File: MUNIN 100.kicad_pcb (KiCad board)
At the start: 2 copper layers, 100 x 75 mm, 78 parts, among them IC1 ACHS-7123, J1 TX_IN, J2 Conn_Coaxial, J3 Conn_01x03_Male, J4 3-647630-4, Q1 ISS55EP06LMXTSA1, Q2 MRF101AN, Q3 MRF101BN, U1 TL783CKTT, U2 LM358

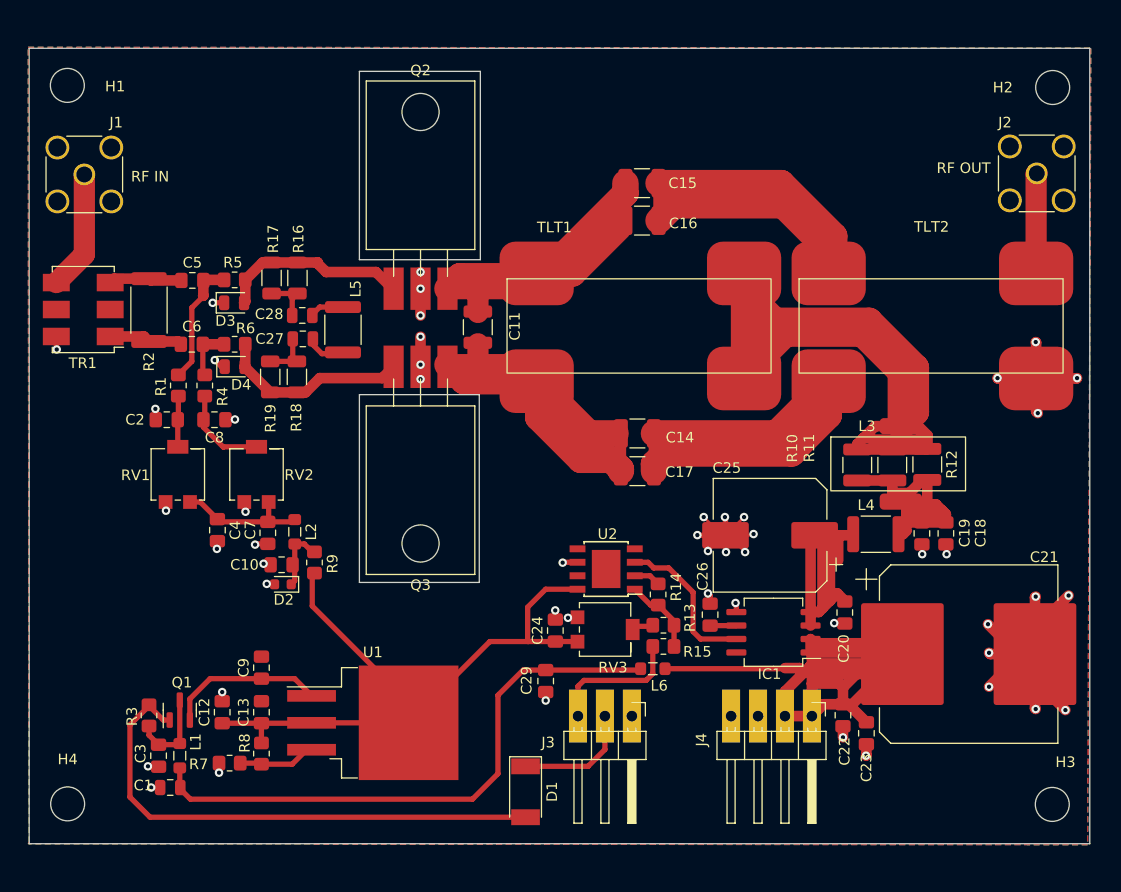
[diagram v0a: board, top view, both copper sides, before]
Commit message: first pcb release
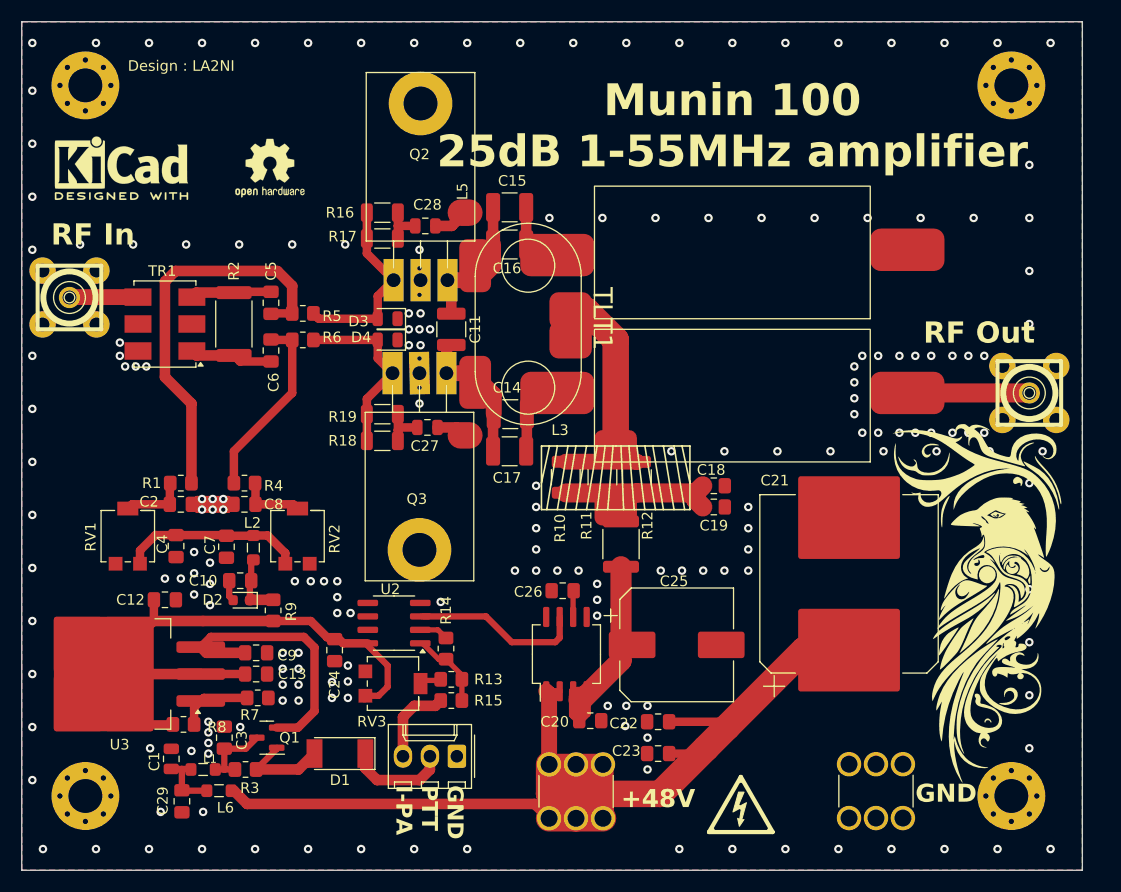
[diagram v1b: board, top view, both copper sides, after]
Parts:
- removed U1: TL783CKTT, Package_TO_SOT_SMD:TO-263-3_TabPin2
- added G***: LOGO, Munin_logo:Munin, F.Cu at (135.0, 130.0)
- added J5: Conn_01x01_Pin, 7461057:7461057, F.Cu at (123.0, 150.1)
- added REF**: OSHW-Logo2_7.3x6mm_SilkScreen, Symbol:OSHW-Logo2_7.3x6mm_SilkScreen, F.Cu at (68.4, 88.8)
- added REF**: Symbol_HighVoltage_Triangle_6x6mm_Copper, logo:Symbol_HighVoltage_Triangle_6x6mm_Copper, F.Cu at (112.8, 148.8)
- added REF**: KiCad-Logo2_5mm_SilkScreen, Symbol:KiCad-Logo2_5mm_SilkScreen, F.Cu at (54.4, 88.8)
- added U3: TL783, Package_TO_SOT_SMD:TO-263-3_TabPin2, F.Cu at (54.2, 136.5)
- H1, H2, H3, H4: value MH -> MountingHole_Pad; footprint MountingHole:MountingHole_3.2mm_M3 -> MountingHole:MountingHole_3.2mm_M3_Pad_Via
- J1, J2: footprint Connector_Coaxial:SMA_Amphenol_132291_Vertical -> SMA_PINS:SMA_PINS
- J3: footprint Connector_PinHeader_2.54mm:PinHeader_1x03_P2.54mm_Horizontal -> Connector_Molex:Molex_KK-254_AE-6410-03A_1x03_P2.54mm_Vertical
- J4: value 3-647630-4 -> Conn_01x01_Pin; footprint Connector_PinHeader_2.54mm:PinHeader_1x04_P2.54mm_Horizontal -> 7461057:7461057
- L1: value L_Core_Ferrite_Small -> 742792096
- L2: value FB -> Wurth: 742792096
- L3: value L_Core_Iron -> FT-50-43; footprint LA2NI:FT_50_1 -> T50:T50_V_smd
- L4: value Ferrite Bead 742792514 -> HI1806T600R-10
- L5: footprint Inductor_SMD:L_1812_4532Metric -> Resistor_THT:R_Axial_DIN0918_L18.0mm_D9.0mm_P30.48mm_Horizontal
- TLT1: value TLT -> FT94-61; footprint LA2NI:TLT_94_3 -> TLT:TLT
- TLT2: value TLT -> FT94-61; footprint LA2NI:TLT_94_3 -> Amidon_Binocular:Dual_FB-61-4852
- U2: footprint Package_SO:Diodes_PSOP-8 -> Package_SO:SOIC-8_3.9x4.9mm_P1.27mm
- moved L6 42.5 mm to (63.6, 147.5)
- moved C29 36.1 mm to (60.1, 148.5)
- moved R10 27.5 mm to (96.3, 117.9)
- moved R12 27.4 mm to (103.0, 118.0)
- moved R11 27.4 mm to (99.8, 117.9)
- moved L3 27.3 mm to (101.0, 118.0)
- moved C20 26.1 mm to (98.6, 140.9), turned to 180 degrees
- moved L4 24.0 mm to (101.5, 124.2), turned to -90 degrees
- moved C18 22.3 mm to (110.2, 118.8), turned to 180 degrees
- moved C24 20.9 mm to (74.5, 134.2), turned to -90 degrees
- moved J2 20.7 mm to (140.0, 110.0), turned to 180 degrees
- moved R13 20.6 mm to (85.5, 137.0)
- moved R14 20.6 mm to (85.0, 134.1)
- moved R15 20.6 mm to (85.5, 139.0)
- moved RV3 20.6 mm to (80.0, 137.4)
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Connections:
- C21 pad 1: Net-(C21-Pad1) -> Net-(J4-Pin_1)
- C22 pad 1: Net-(C21-Pad1) -> Net-(J4-Pin_1)
- C23 pad 1: Net-(C21-Pad1) -> Net-(J4-Pin_1)
- IC1 pad 1: Net-(C21-Pad1) -> Net-(J4-Pin_1)
- IC1 pad 2: Net-(C21-Pad1) -> Net-(J4-Pin_1)
- J4 pad 1: Net-(C21-Pad1) -> Net-(J4-Pin_1)
- L6 pad 2: Net-(C21-Pad1) -> Net-(J4-Pin_1)
- Q2 pad : (no net) -> GND
- Q3 pad : (no net) -> GND
- RV2 pad 1: Net-(C4-Pad1) -> GND
- RV2 pad 3: GND -> Net-(C4-Pad1)
- TLT2 pad 1: Net-(C15-Pad2) -> Net-(C14-Pad2)
- TLT2 pad 4: Net-(C14-Pad2) -> Net-(C15-Pad2)
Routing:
- net Net-(J4-Pin_1): track 0.00 -> 120.6 mm
- net Net-(C21-Pad1): track 87.1 -> 0.00 mm
- net GND: track 106.1 -> 23.6 mm, vias 51 -> 190
- net Net-(L3-Pad1): track 94.8 -> 22.1 mm
- net +48V: track 55.2 -> 6.25 mm
- net Net-(C15-Pad2): track 46.5 -> 3.50 mm
- net Net-(D1-A): track 49.9 -> 8.97 mm
- net Net-(C14-Pad2): track 44.4 -> 3.53 mm
- net Net-(Q3-D): track 47.2 -> 13.5 mm
- net Net-(Q2-D): track 46.7 -> 13.2 mm
- net Net-(C5-Pad2): track 11.8 -> 37.6 mm
- net Net-(C18-Pad2): track 29.2 -> 14.8 mm
- net Net-(C6-Pad2): track 4.96 -> 17.8 mm
- net Net-(Q1-S): track 14.9 -> 26.2 mm
- net +5V: track 65.1 -> 55.3 mm
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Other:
- board size 100 x 75 mm -> 100 x 80 mm
- board text added: "+48V"
- board text added: "Design : LA2NI"
- board text added: "GND"
- board text added: "GND PTT I-PA"
- board text added: "Munin 100 25dB 1-55MHz amplifier"
- board text added: "RF In"
- board text added: "RF Out"
- board text removed: "RF IN"
- board text removed: "RF OUT"
